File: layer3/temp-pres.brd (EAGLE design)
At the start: 9 parts, among them U1 TMP1021:1, U2 MS5803-14BA

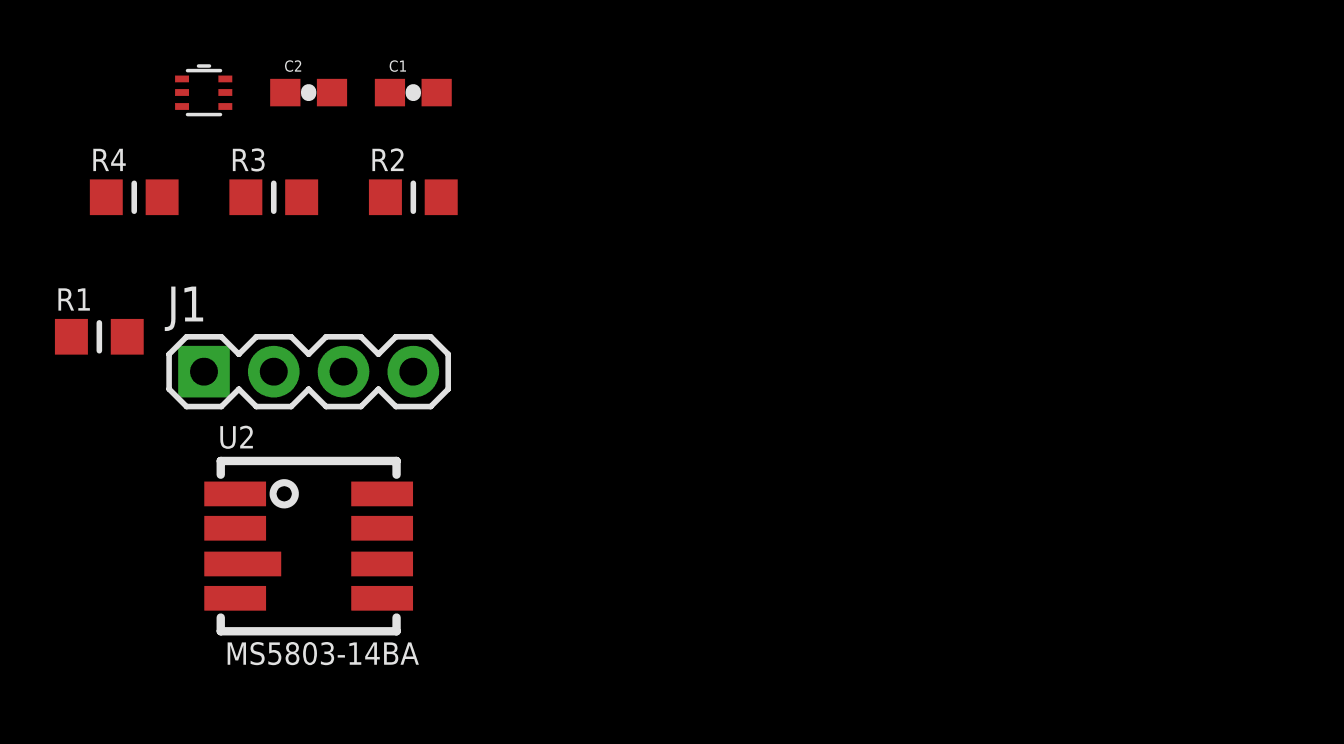
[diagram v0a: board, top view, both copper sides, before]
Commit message: intital board layout
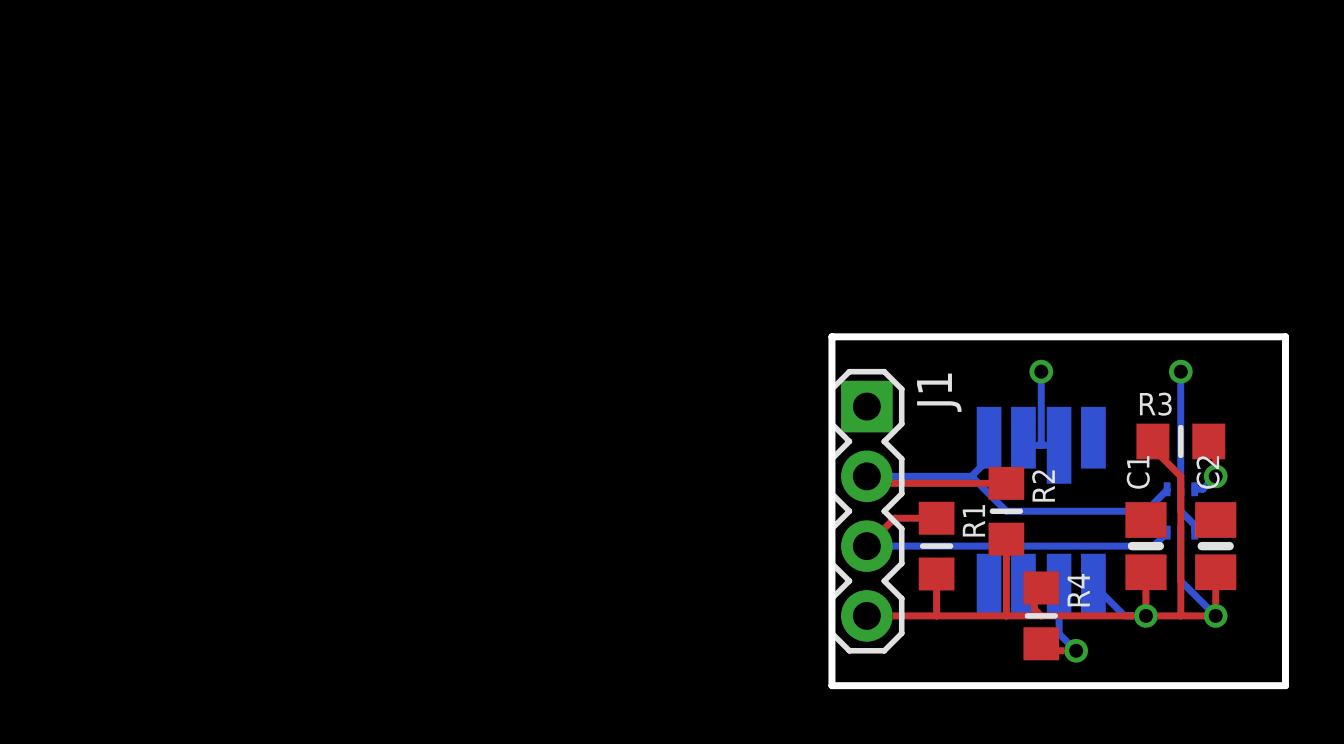
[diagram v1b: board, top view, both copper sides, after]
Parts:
- C1: device SparkFun:0603-CAP -> microbuilder:0805-NO
- C2: device SparkFun-Capacitors:0603-CAP -> microbuilder:0805-NO
- moved U1 38.7 mm to (12.7, 6.35), flipped to the bottom, turned to 270 degrees
- moved C2 36.9 mm to (14.0, 5.08), turned to 90 degrees
- moved R4 36.4 mm to (7.62, 2.54), turned to 270 degrees
- moved R3 34.2 mm to (12.7, 8.89)
- moved R1 31.4 mm to (3.81, 5.08), turned to 270 degrees
- moved C1 31.4 mm to (11.4, 5.08), turned to 90 degrees
- moved U2 26.7 mm to (7.62, 6.35), flipped to the bottom, turned to 270 degrees
- moved R2 24.4 mm to (6.35, 6.35), turned to 270 degrees
- moved J1 24.2 mm to (1.27, 10.2), turned to 270 degrees
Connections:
- removed net ALERT: R3.2
- new net N$1: R3.2, U1.3
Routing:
- net +3V3: track 0.00 -> 34.6 mm, vias 0 -> 2
- net SCL: track 0.00 -> 18.7 mm
- net SDA: track 0.00 -> 15.8 mm
- net GND: track 0.00 -> 10.7 mm, vias 0 -> 2
- net PS: track 0.00 -> 4.04 mm, vias 0 -> 1
- net N$1: track 0.00 -> 2.33 mm, vias 0 -> 1
- added copper zone on layer 1, net GND
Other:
- board outline added: 16.5 x 12.7 mm
